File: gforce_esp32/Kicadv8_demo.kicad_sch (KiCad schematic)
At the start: 26 parts, among them J1 USB_C_Receptacle, SW1 TL3215AF160BQ, SW2 TL3215AF160RQ, U1 ESP32-S3-MINI-1U, U2 AP2112K-3.3, U3 LIS3DH

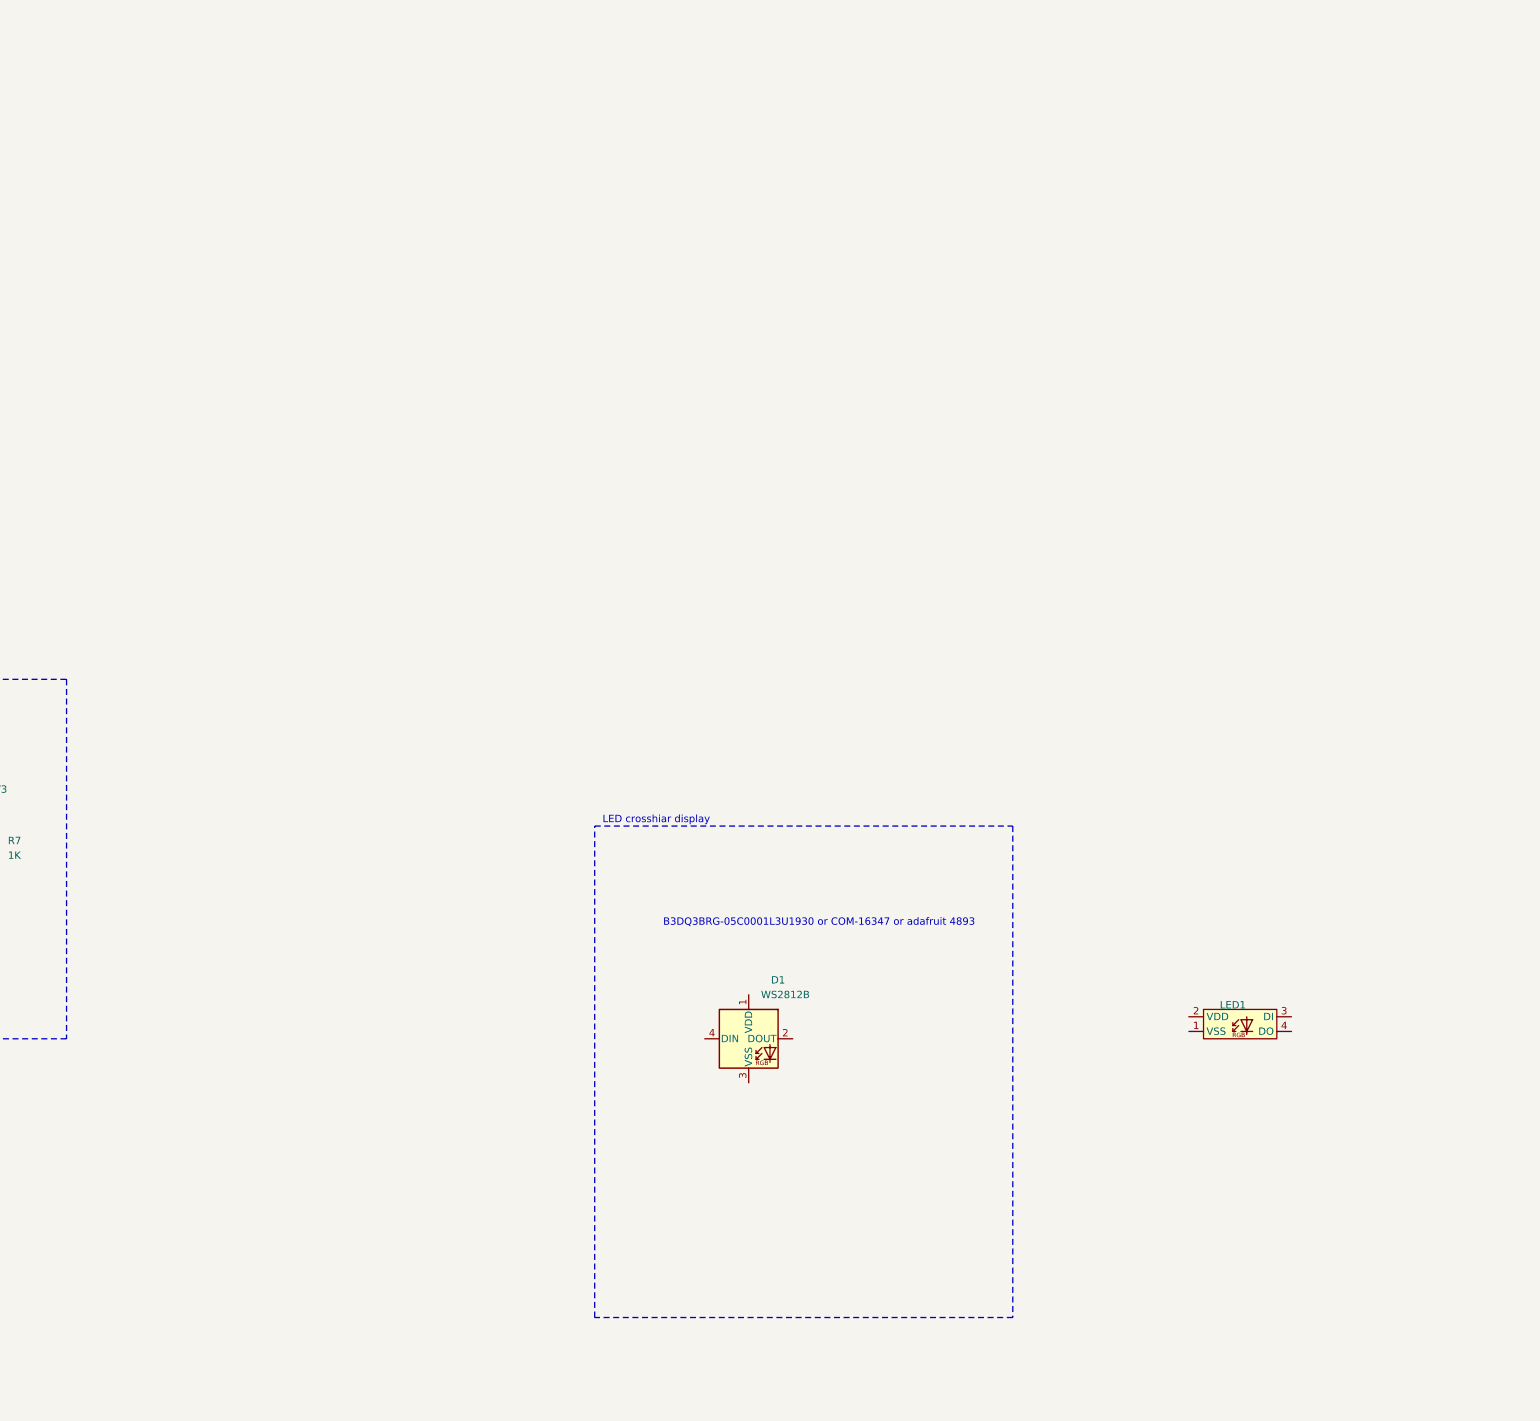
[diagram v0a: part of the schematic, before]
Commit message: layout placing parts
lined up leds
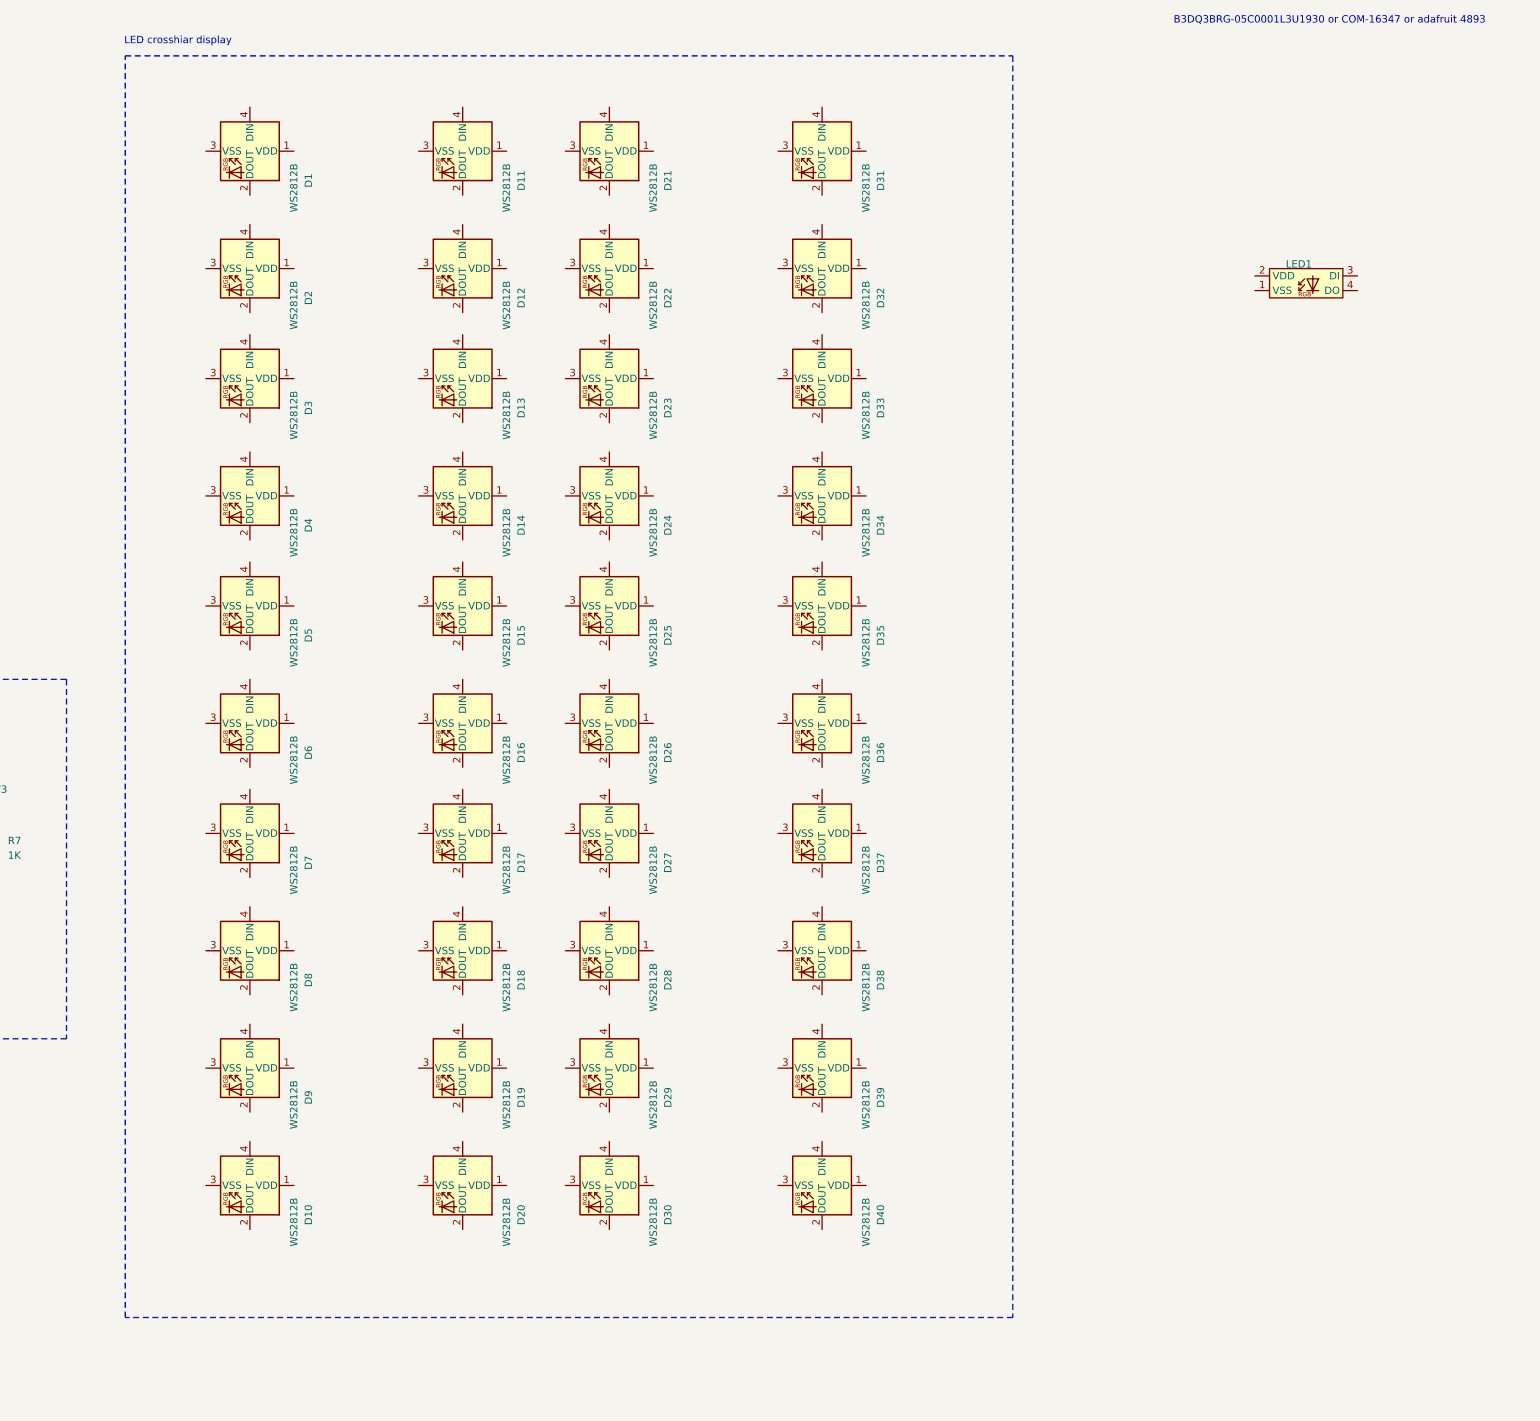
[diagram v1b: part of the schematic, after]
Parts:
- added D10, D11, D12, D13, D14, D15, D16, D17, D18, D19, D2, D20, D21, D22, D23, D24, D25, D26, D27, D28, D29, D3, D30, D31, D32, D33, D34, D35, D36, D37, D38, D39, D4, D40, D5, D6, D7, D8, D9: WS2812B, LED_SMD:LED_WS2812B_PLCC4_5.0x5.0mm_P3.2mm, symbol LED:WS2812B
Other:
- moved on the sheet: D1, LED1
